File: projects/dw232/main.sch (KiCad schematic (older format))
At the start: 2 parts, among them P101 CONN_01X07

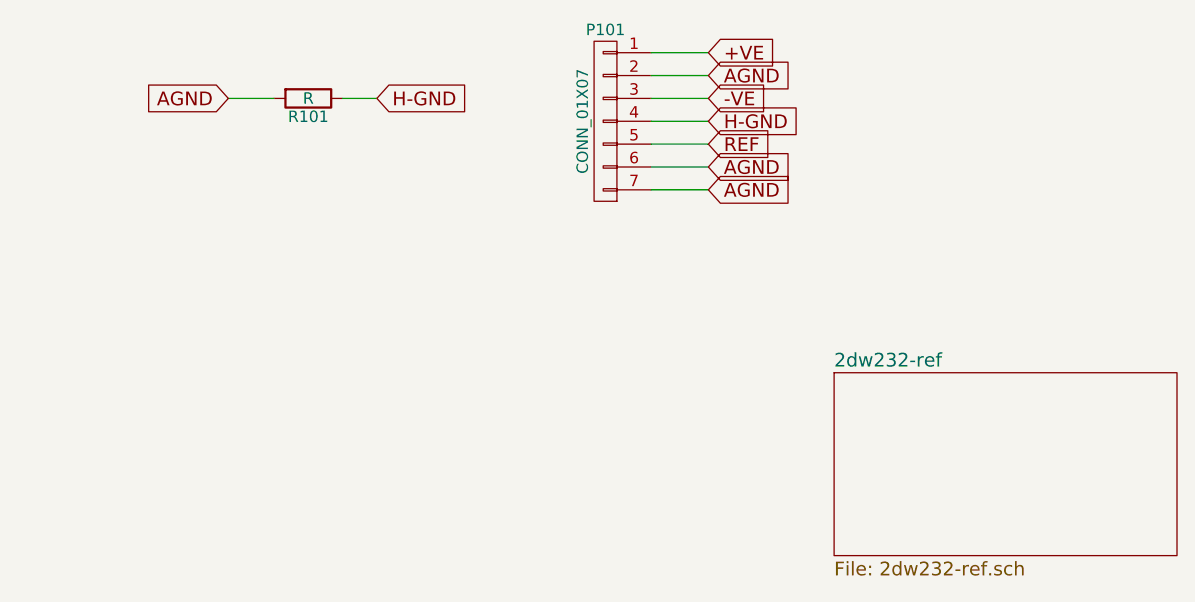
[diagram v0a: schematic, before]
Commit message: v0.2 2dw232
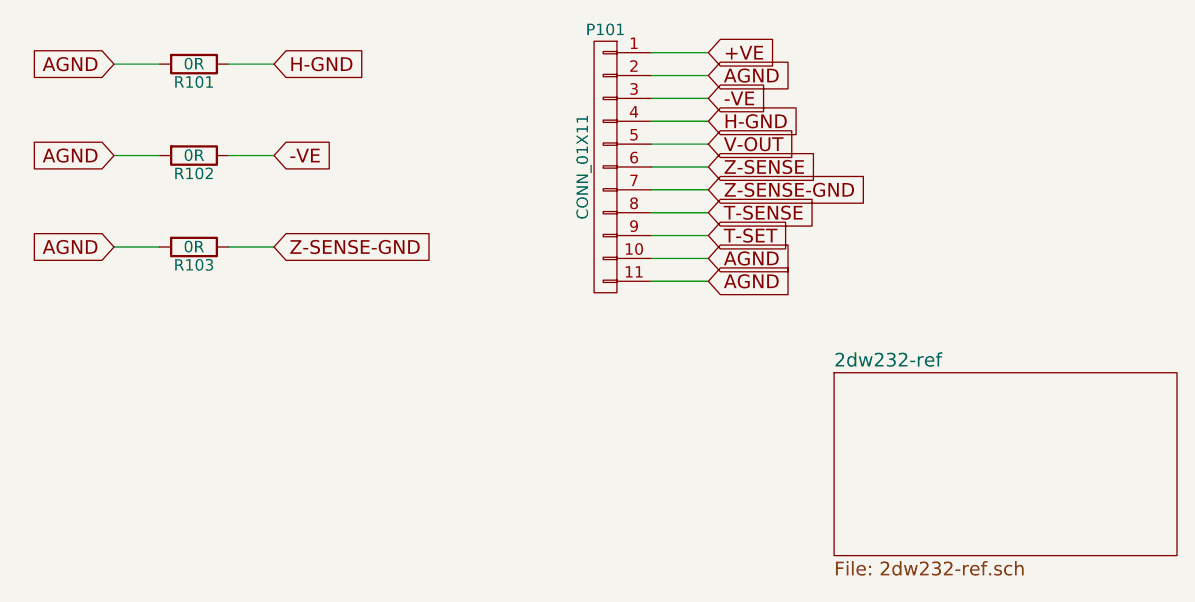
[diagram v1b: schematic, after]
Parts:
- removed P101: CONN_01X07, Pin_Headers:Pin_Header_Straight_1x07, symbol CONN_01X07
- added P101: CONN_01X11, symbol CONN_01X11
- added R102, R103: 0R, symbol R
- R101: value R -> 0R
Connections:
- net +VE: now also P101.1 (P1)
- net -VE: now also P101.3 (P3), R102.1
- net AGND: now also P101.10 (P10), P101.11 (P11), P101.2 (P2), R102.2, R103.2
- net H-GND: now also P101.4 (P4)
- new net T-SENSE: P101.8 (P8)
- new net T-SET: P101.9 (P9)
- new net V-OUT: P101.5 (P5)
- new net Z-SENSE: P101.6 (P6)
- new net Z-SENSE-GND: P101.7 (P7), R103.1
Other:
- moved on the sheet: R101
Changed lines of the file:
@@
 F1 "2dw232-ref.sch" 60
 $EndSheet
-$Comp
-L CONN_01X07 P101
-U 1 1 58A3916C
-P 4200 1750
-F 0 "P101" H 4200 2150 50  0000 C CNN
-F 1 "CONN_01X07" V 4300 1750 50  0000 C CNN
-F 2 "Pin_Headers:Pin_Header_Straight_1x07" H 4200 1750 50  0001 C CNN
-F 3 "" H 4200 1750 50  0000 C CNN
-	1    4200 1750
-	-1   0    0    -1
-$EndComp
 Text GLabel 4650 1450 2    60   Input ~ 0
 +VE
@@
 Wire Wire Line
 	4400 1550 4650 1550
+Text GLabel 4650 1950 2    60   Input ~ 0
+Z-SENSE
 Text GLabel 4650 1850 2    60   Input ~ 0
-REF
-Text GLabel 4650 1950 2    60   Input ~ 0
-AGND
-Text GLabel 4650 2050 2    60   Input ~ 0
-AGND
+V-OUT
+Text GLabel 4650 2150 2    60   Input ~ 0
+T-SENSE
 Wire Wire Line
-	4400 1950 4650 1950
-Wire Wire Line
-	4400 2050 4650 2050
+	4400 2150 4650 2150
 Text GLabel 4650 1650 2    60   Input ~ 0
 -VE
@@
 	4400 1750 4650 1750
 Wire Wire Line
-	4400 1850 4650 1850
-Text GLabel 3200 1650 2    60   Input ~ 0
+	4400 1950 4650 1950
+Text GLabel 2750 1500 2    60   Input ~ 0
 H-GND
-Text GLabel 2550 1650 0    60   Input ~ 0
+Text GLabel 2050 1500 0    60   Input ~ 0
 AGND
 $Comp
 L R R101
 U 1 1 58A39183
-P 2900 1650
-F 0 "R101" V 2980 1650 50  0000 C CNN
-F 1 "R" V 2900 1650 50  0000 C CNN
-F 2 "Resistors_SMD:R_1206" V 2830 1650 50  0001 C CNN
-F 3 "" H 2900 1650 50  0000 C CNN
-	1    2900 1650
+P 2400 1500
+F 0 "R101" V 2480 1500 50  0000 C CNN
+F 1 "0R" V 2400 1500 50  0000 C CNN
+F 2 "Resistors_SMD:R_1206" V 2330 1500 50  0001 C CNN
+F 3 "" H 2400 1500 50  0000 C CNN
+	1    2400 1500
 	0    1    1    0
 $EndComp
 Wire Wire Line
-	2550 1650 2750 1650
+	2050 1500 2250 1500
 Wire Wire Line
-	3050 1650 3200 1650
+	2550 1500 2750 1500
+$Comp
+L R R102
+U 1 1 58B28AD9
+P 2400 1900
+F 0 "R102" V 2480 1900 50  0000 C CNN
+F 1 "0R" V 2400 1900 50  0000 C CNN
+F 2 "" V 2330 1900 50  0000 C CNN
+F 3 "" H 2400 1900 50  0000 C CNN
+	1    2400 1900
+	0    1    1    0
+$EndComp
+Text GLabel 2750 1900 2    60   Input ~ 0
+-VE
+Wire Wire Line
+	2550 1900 2750 1900
+Text GLabel 2050 1900 0    60   Input ~ 0
+AGND
+Wire Wire Line
+	2050 1900 2250 1900
+Text GLabel 4650 2250 2    60   Input ~ 0
+T-SET
+Text GLabel 4650 2350 2    60   Input ~ 0
+AGND
+Text GLabel 4650 2450 2    60   Input ~ 0
+AGND
+$Comp
+L CONN_01X11 P101
+U 1 1 58B28D45
+P 4200 1950
+F 0 "P101" H 4200 2550 50  0000 C CNN
+F 1 "CONN_01X11" V 4300 1950 50  0000 C CNN
+F 2 "" H 4200 1950 50  0000 C CNN
+F 3 "" H 4200 1950 50  0000 C CNN
+	1    4200 1950
+	-1   0    0    -1
+$EndComp
+Wire Wire Line
+	4400 2250 4650 2250
+Wire Wire Line
+	4400 2350 4650 2350
+Wire Wire Line
+	4400 2450 4650 2450
+Text GLabel 4650 2050 2    60   Input ~ 0
+Z-SENSE-GND
+Wire Wire Line
+	4400 2050 4650 2050
+Wire Wire Line
+	4400 1850 4650 1850
+$Comp
+L R R103
+U 1 1 58B32019
+P 2400 2300
+F 0 "R103" V 2480 2300 50  0000 C CNN
+F 1 "0R" V 2400 2300 50  0000 C CNN
+F 2 "" V 2330 2300 50  0000 C CNN
+F 3 "" H 2400 2300 50  0000 C CNN
+	1    2400 2300
+	0    1    1    0
+$EndComp
+Text GLabel 2750 2300 2    60   Input ~ 0
+Z-SENSE-GND
+Wire Wire Line
+	2550 2300 2750 2300
+Text GLabel 2050 2300 0    60   Input ~ 0
+AGND
+Wire Wire Line
+	2050 2300 2250 2300
 $EndSCHEMATC
